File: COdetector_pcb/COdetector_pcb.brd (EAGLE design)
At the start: 42 parts

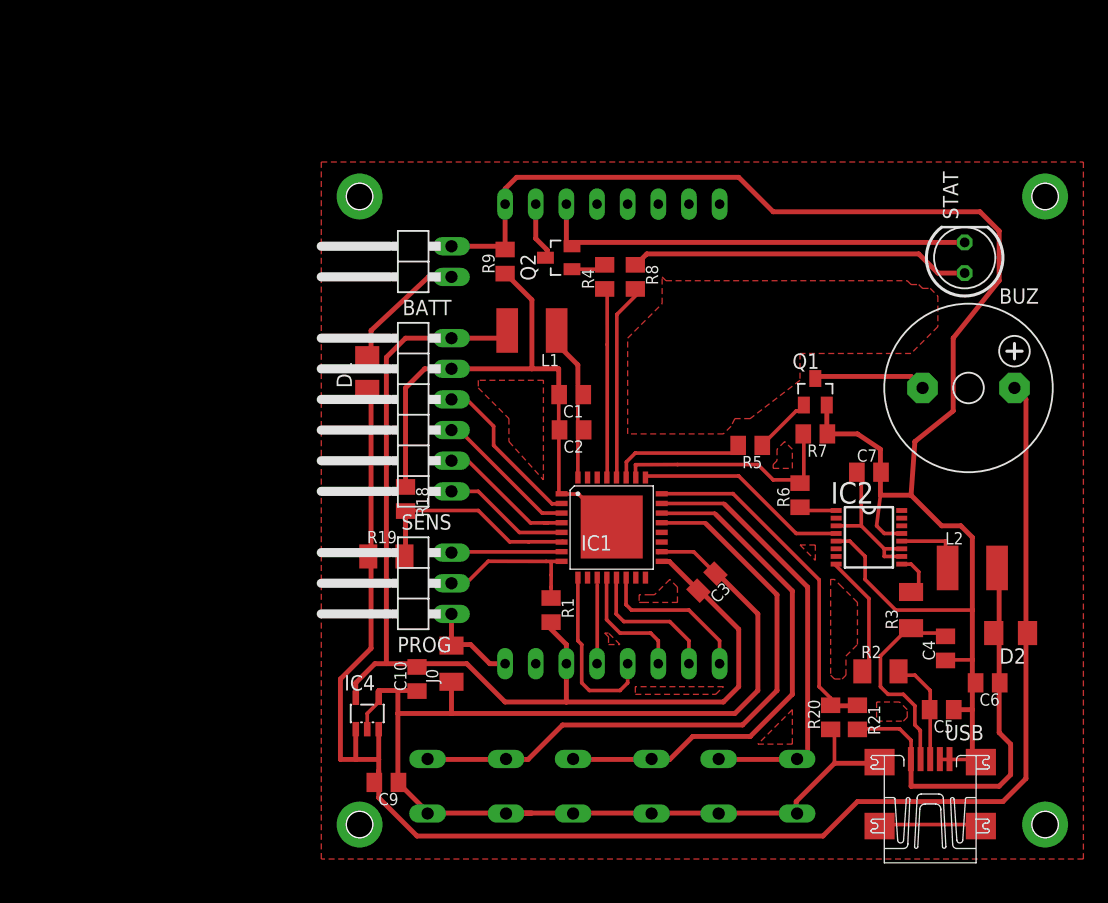
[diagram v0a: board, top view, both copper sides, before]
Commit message: Doone, checked, ready
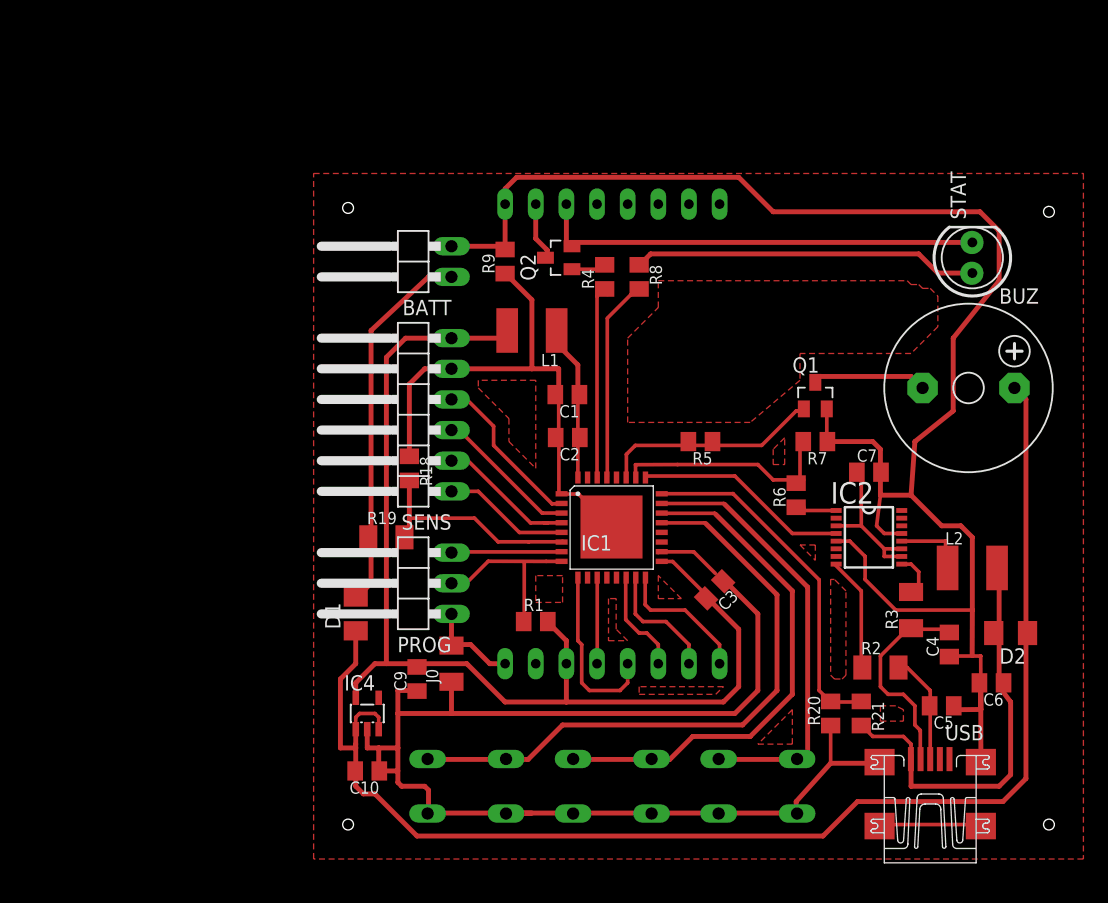
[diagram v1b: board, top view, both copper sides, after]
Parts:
- moved D1 20.0 mm to (25.4, 20.0)
- moved C9 8.94 mm to (30.5, 14.6), turned to 90 degrees
- moved C10 8.67 mm to (26.4, 6.99), turned to 180 degrees
- moved R5 4.14 mm to (54.0, 34.3)
- moved R18 2.56 mm to (29.8, 32.1)
- moved R1 1.59 mm to (40.3, 19.4), turned to 0 degrees
- moved R19 1.59 mm to (27.9, 26.4)
- moved C3 0.90 mm to (55.2, 22.0)
- moved C2 0.71 mm to (43.0, 34.6)
- moved STAT 0.64 mm to (76.5, 49.5)
- moved R7 0.63 mm to (63.5, 34.3)
- moved C4 0.45 mm to (74.6, 17.5)
- moved R21 0.45 mm to (67.3, 11.7)
- moved R8 0.32 mm to (48.9, 47.9)
- moved R2 0.32 mm to (68.9, 15.6)
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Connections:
- new net S$81: C2.1, C2.2
- net GND: now also C9.1, R20.1; no longer C10.1, Q1.2
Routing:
- net S$73: track 40.1 -> 13.5 mm
- net S$31: track 10.0 -> 30.6 mm
- net S$86: track 0.00 -> 15.5 mm
- net S$57: track 15.5 -> 0.09 mm
- net GND: track 263.7 -> 275.4 mm, vias 4 -> 0
- net S$64: track 10.2 -> 17.5 mm
- net S$8: track 3.91 -> 0.00 mm
- net S$74: track 0.00 -> 2.80 mm
- net S$3: track 13.4 -> 11.0 mm
- net S$55: track 30.3 -> 28.0 mm
- net S$62: track 2.30 -> 0.00 mm, vias 0 -> 1
- net S$9: track 2.74 -> 4.57 mm
- net S$1: track 10.5 -> 8.77 mm
- net S$2: track 12.1 -> 10.4 mm
- net S$28: track 6.11 -> 4.52 mm
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- added copper zone on layer 1, net S$8
- added copper zone on layer 1, net S$84
- added copper zone on layer 1, net S$87
- added copper zone on layer 1, net S$88
- removed copper zone on layer 1, net S$74
- removed copper zone on layer 1, net S$81
- removed copper zone on layer 1, net S$83

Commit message: V3 RC
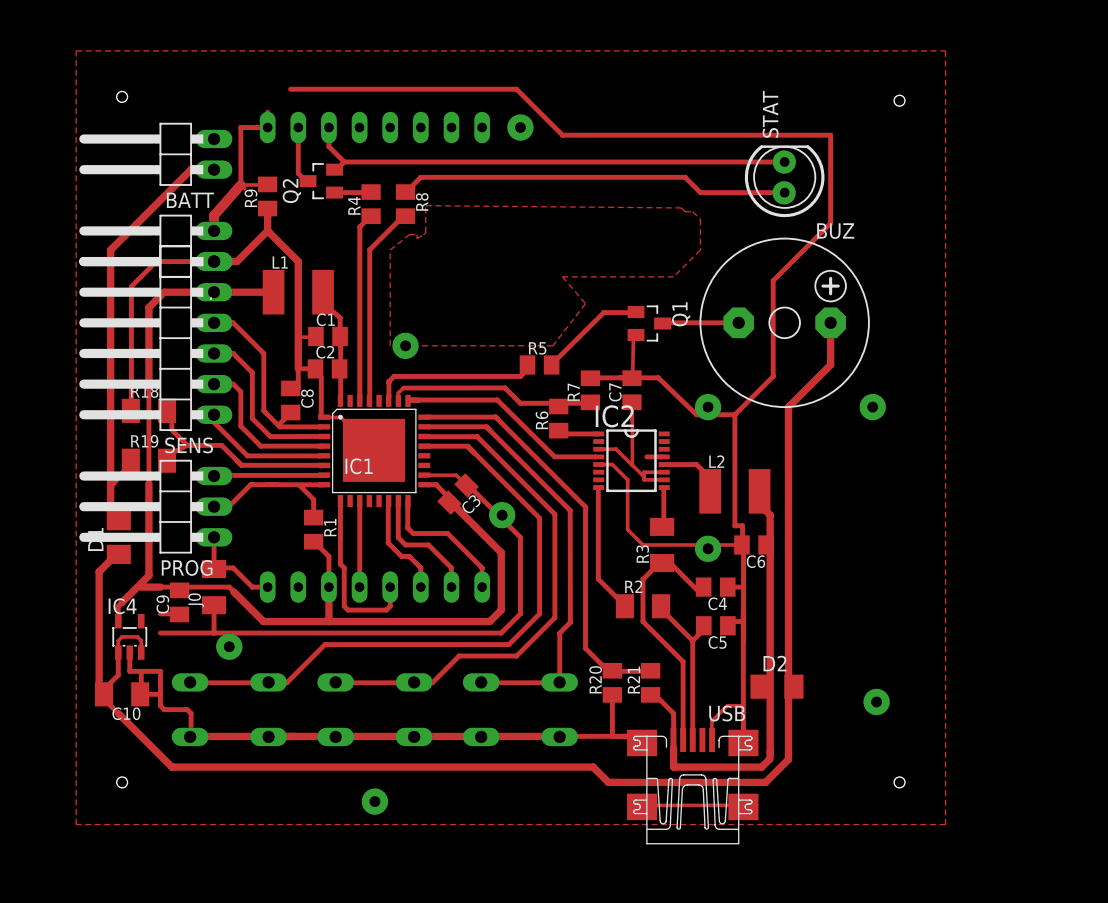
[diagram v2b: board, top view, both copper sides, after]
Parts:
- added .: (no value), pinhead:1X02/90
- added C8: (no value), ref-packages:C0805K
- C10, R18: device ref-packages:C0805K -> ref-packages:C1206K
- R19: device ref-packages-longpad:C1206K -> ref-packages:C1206K
- moved C6 22.8 mm to (58.4, 25.7)
- moved C3 22.7 mm to (33.9, 29.9)
- moved R18 22.1 mm to (8.25, 36.8), turned to 0 degrees
- moved BATT 21.6 mm to (9.84, 58.1)
- moved R3 21.3 mm to (50.8, 25.7)
- moved C10 21.3 mm to (6.03, 13.3)
- moved C7 20.8 mm to (48.3, 38.5), turned to 90 degrees
- moved C2 20.7 mm to (23.1, 40.3), turned to 0 degrees
- moved L2 20.7 mm to (56.8, 30.2)
- moved C9 20.7 mm to (10.8, 21.0)
- moved IC1 20.7 mm to (26.9, 33.5)
- moved PROG 20.7 mm to (9.84, 28.9)
- moved R19 20.7 mm to (8.26, 32.7)
- moved R6 20.7 mm to (42.2, 36.2)
- moved S1 20.7 mm to (14.9, 12.1)
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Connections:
- removed net S$20: BUZ.-
- removed net S$35: SENS.6
- removed net S$55: SENS.5
- removed net S$70: STAT.K
- removed net S$76: SENS.1
- removed net S$78: SENS.3
- removed net S$79: SENS.4
- new net S$36: SENS.2
- new net S$50: SENS.3
- new net S$54: SENS.4
- new net S$64: BUZ.-
- new net S$69: IC2.13
- net GND: now also ..2, Q1.2
- net S$31: now also SENS.5; no longer BATT.1
- net S$56: now also STAT.K; no longer E$2.P06
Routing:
- net GNDA: track 0.00 -> 38.9 mm
- net S$56: track 3.49 -> 40.0 mm
- net S$28: track 4.52 -> 37.1 mm
- net S$63: track 4.13 -> 36.0 mm
- net S$55: track 28.0 -> 0.12 mm
- net S$35: track 36.2 -> 10.7 mm
- net S$70: track 33.3 -> 13.4 mm
- net S$99: track 0.00 -> 17.8 mm
- net S$89: track 0.00 -> 17.0 mm
- net S$96: track 0.00 -> 15.5 mm
- net S$31: track 30.6 -> 46.0 mm
- net S$54: track 0.00 -> 15.3 mm
- net S$6: track 27.7 -> 13.2 mm
- net S$50: track 0.00 -> 14.0 mm
- net S$86: track 15.5 -> 29.1 mm
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- removed copper zone on layer 1, net S$34
- removed copper zone on layer 1, net S$50
- removed copper zone on layer 1, net S$54
- removed copper zone on layer 1, net S$65
- removed copper zone on layer 1, net S$67
- removed copper zone on layer 1, net S$8
- removed copper zone on layer 1, net S$82
- removed copper zone on layer 1, net S$84
- removed copper zone on layer 1, net S$87
- removed copper zone on layer 1, net S$88

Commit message: Before sec version with all put togehter
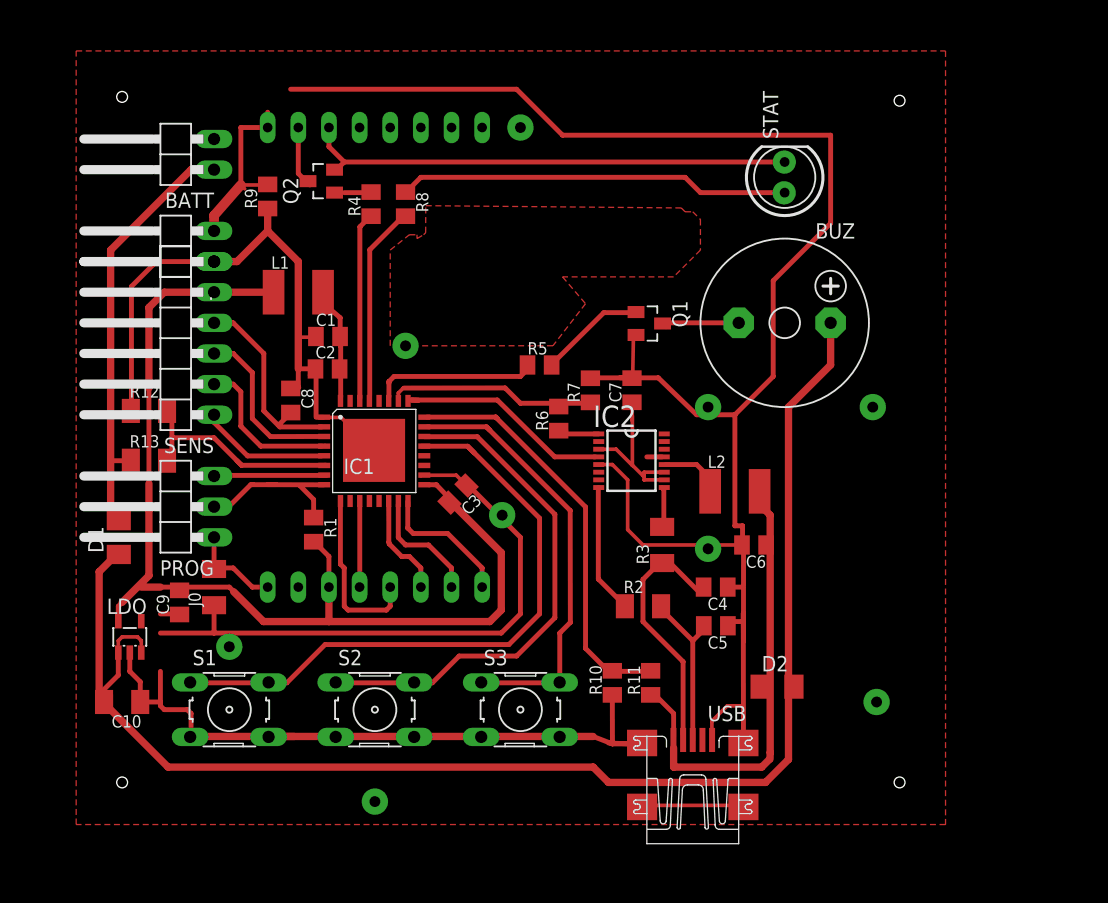
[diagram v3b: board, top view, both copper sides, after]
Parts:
- moved C10 0.64 mm to (6.03, 12.7)
- flipped S1 to the top
- flipped S2 to the top
- flipped S3 to the top
- renumbered IC4 to LDO, R18 to R12, R19 to R13, R20 to R10, R21 to R11
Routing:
- net GND: track 282.0 -> 278.3 mm
- net S$85: track 0.00 -> 3.01 mm
- net S$63: track 36.0 -> 35.3 mm
- net S$87: track 0.00 -> 0.58 mm

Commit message: New Version, final
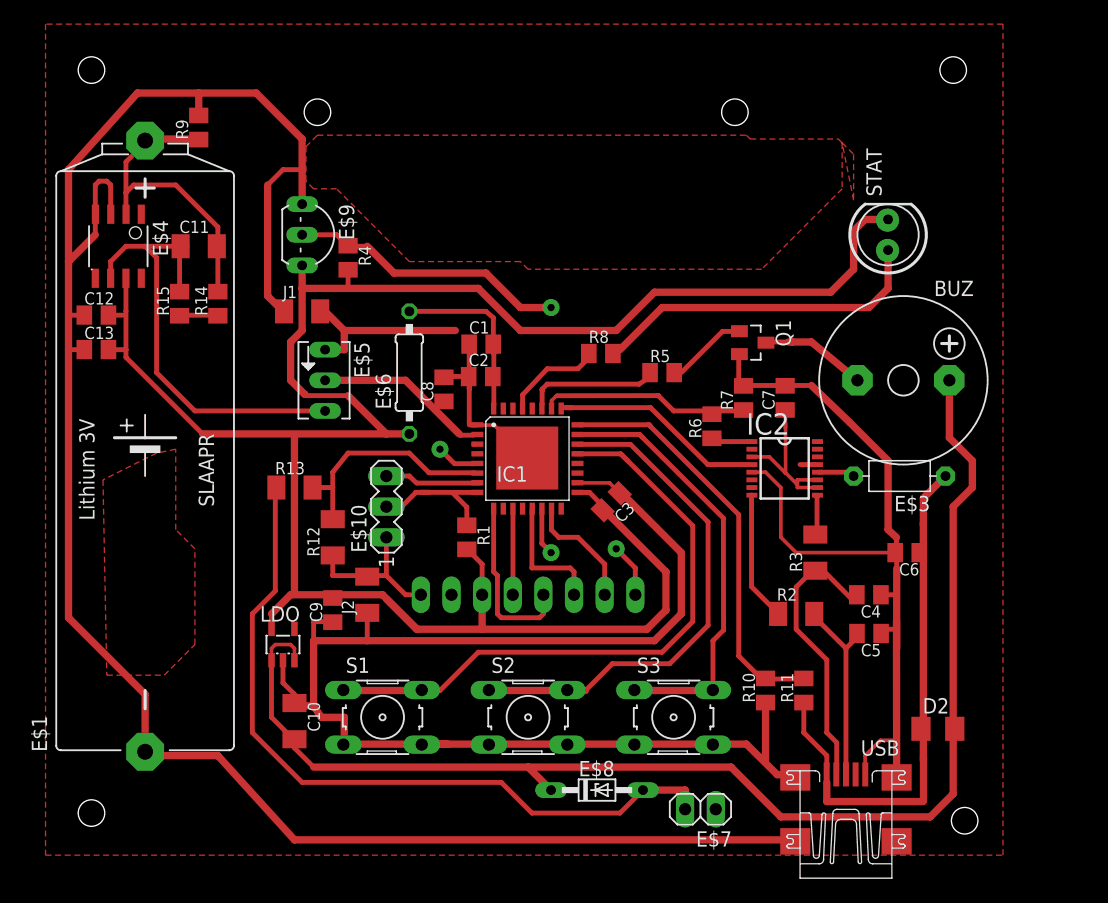
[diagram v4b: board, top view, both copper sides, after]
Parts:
- removed ., BATT: (no value), pinhead:1X02/90
- removed D1: (no value), rcl:M1206
- removed J0: (no value), ref-packages-longpad:C1206K
- removed L1, L2: (no value), ref-packages:C1812K
- removed PROG: (no value), pinhead:1X03/90
- removed Q2: (no value), avago:SOT23
- removed SENS: (no value), pinhead:1X06/90
- added C11, J1: (no value), ref-packages:C1206K
- added C12, C13, R14, R15: (no value), ref-packages:C0805K
- added E$1: (no value), battery:SL-160AA/PR
- added E$10: (no value), con-lstb:MA03-1
- added E$3: (no value), discrete:R-7,5
- added E$4: (no value), atmel:8S1
- added E$5: (no value), pot:B64Y
- added E$6: (no value), ref-packages:0207/10
- added E$7: (no value), pinhead:1X02
- added E$8: (no value), diode:DO34Z7
- added E$9: (no value), ref-packages:TO92-LINE
- added J2: (no value), ref-packages-longpad:C1206K
- E$2: device 3310LCD:3310 -> con-lstb:MA08-1
- moved E$2 23.4 mm to (39.7, 21.6)
- moved R8 20.4 mm to (45.7, 41.6), turned to 0 degrees
- moved R12 18.5 mm to (23.5, 26.4), turned to 90 degrees
- moved C10 14.4 mm to (20.3, 11.1), turned to 270 degrees
- moved D2 13.8 mm to (73.7, 10.5)
- moved USB 13.0 mm to (66.0, 4.45)
- moved C8 12.7 mm to (32.7, 38.6), turned to 90 degrees
- moved C3 12.7 mm to (46.6, 29.3)
- moved C5 12.7 mm to (68.0, 18.4)
- moved IC1 12.7 mm to (39.6, 32.9)
- moved IC2 12.7 mm to (61.0, 32.1)
- moved R10 12.7 mm to (59.4, 13.7)
- moved R11 12.7 mm to (62.5, 13.7)
- moved R2 12.7 mm to (61.9, 20.0)
- moved R3 12.7 mm to (63.5, 25.1)
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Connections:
- removed net S$14: PROG.3
- removed net S$19: STAT.A
- removed net S$2: E$2.P12
- removed net S$3: E$2.P11
- removed net S$31: SENS.5
- removed net S$36: SENS.2
- removed net S$4: E$2.P15
- removed net S$41: E$2.P16
- removed net S$5: E$2.P14
- removed net S$50: SENS.3
- removed net S$53: E$2.P07
- removed net S$64: BUZ.-
- removed net S$7: PROG.2
- removed net S$81: C2.1, C2.2
- new net S$102: E$3.1
- new net S$106: E$10.3
- new net S$108: E$8.C
- new net S$111: R10.1
- new net S$18: E$6.2
- new net S$22: E$3.2
- new net S$55: STAT.A
- new net S$57: E$2.3
- new net S$62: E$9.1, STAT.K
- new net S$71: E$5.S
- new net S$8: Q1.2
- new net S$84: E$6.1
- new net S$86: E$9.2
- net GND: now also C1.1, E$1.-, E$10.1, E$2.8, E$5.E, E$7.1, E$9.3, J2.1, J2.2, R12.1; no longer ..2, BATT.2, E$2.P08, E$2.P18, J0.1, J0.2, PROG.1, Q1.2, R10.1
- net S$1: now also C2.1, C2.2; no longer E$2.P13
- net S$44: now also E$5.A; no longer BUZ.+
- net S$54: now also E$7.2, E$8.A; no longer SENS.4
- net S$56: now also BUZ.-; no longer STAT.K
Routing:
- net GND: track 278.3 -> 375.4 mm, vias 9 -> 0
- net S$62: track 0.00 -> 68.9 mm, vias 1 -> 0
- net S$108: track 0.00 -> 63.3 mm
- net S$30: track 58.1 -> 2.88 mm
- net S$54: track 15.3 -> 62.1 mm
- net S$31: track 46.0 -> 2.86 mm
- net S$84: track 1.14 -> 41.7 mm
- net GNDA: track 38.9 -> 0.00 mm
- net S$19: track 31.6 -> 0.00 mm
- net S$56: track 40.0 -> 8.77 mm
- net S$100: track 0.00 -> 29.4 mm
- net S$63: track 35.3 -> 7.80 mm, vias 0 -> 2
- net S$55: track 0.12 -> 27.5 mm
- net S$86: track 29.1 -> 4.20 mm
- net S$88: track 0.00 -> 21.2 mm
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- added copper zone on layer 1, net S$76
- added copper zone on layer 1, net S$83
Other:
- board text added: "CO MONITOR by A. Tyran AGH WIEiT Kraków 2015"
- board text added: "TGS5042"
- board text removed: "2015"
- board text removed: "A.Tyran"
- board text removed: "CO detector"
